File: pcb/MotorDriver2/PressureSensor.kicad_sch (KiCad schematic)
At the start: 22 parts, among them J2 Conn_01x02, J3 Conn_01x02, J4 Conn_01x02, J5 Conn_01x02, U6 LM324DR

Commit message: Laying out PCB
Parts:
- C_A1: LCSC (none) -> C77012
- R18, R19: LCSC (none) -> C25871
- U6: footprint footprintLib:D14 -> CapstoneFootprints:D14
- VR1, VR2, VR3, VR4: footprint footprintLib:TS53YJ105MR10 -> CapstoneFootprints:TS53YJ105MR10
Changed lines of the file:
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@@
 		(dnp no)
 		(fields_autoplaced yes)
-		(property "Reference" "#PWR065"
+		(property "Reference" "#PWR025"
 			(at 60.96 111.76 0)
 			(effects
@@
 			(project "MotorDriver1"
 				(path "/6e0510ec-6dbc-4bc1-a315-3680b1127a92/84d965bc-7f0b-4bc5-931c-8ce848efd12b"
-					(reference "#PWR065")
+					(reference "#PWR025")
 					(unit 1)
 				)
@@
 		(dnp no)
 		(fields_autoplaced yes)
-		(property "Reference" "#PWR042"
+		(property "Reference" "#PWR026"
 			(at 60.96 171.45 0)
 			(effects
@@
 			(project "MotorDriver1"
 				(path "/6e0510ec-6dbc-4bc1-a315-3680b1127a92/84d965bc-7f0b-4bc5-931c-8ce848efd12b"
-					(reference "#PWR042")
+					(reference "#PWR026")
 					(unit 1)
 				)
@@
 			)
 		)
+		(property "LCSC" "C25871"
+			(at 118.11 39.37 0)
+			(effects
+				(font
+					(size 1.27 1.27)
+				)
+				(hide yes)
+			)
+		)
 		(pin "2"
 		)
@@
 		(dnp no)
 		(fields_autoplaced yes)
-		(property "Reference" "#PWR062"
+		(property "Reference" "#PWR029"
 			(at 185.42 40.64 0)
 			(effects
@@
 			(project "MotorDriver1"
 				(path "/6e0510ec-6dbc-4bc1-a315-3680b1127a92/84d965bc-7f0b-4bc5-931c-8ce848efd12b"
-					(reference "#PWR062")
+					(reference "#PWR029")
 					(unit 1)
 				)
@@
 		(dnp no)
 		(fields_autoplaced yes)
-		(property "Reference" "#PWR064"
+		(property "Reference" "#PWR023"
 			(at 52.07 77.47 0)
 			(effects
@@
 			(project "MotorDriver1"
 				(path "/6e0510ec-6dbc-4bc1-a315-3680b1127a92/84d965bc-7f0b-4bc5-931c-8ce848efd12b"
-					(reference "#PWR064")
+					(reference "#PWR023")
 					(unit 1)
 				)
@@
 		(dnp no)
 		(fields_autoplaced yes)
-		(property "Reference" "#PWR041"
+		(property "Reference" "#PWR024"
 			(at 52.07 137.16 0)
 			(effects
@@
 			(project "MotorDriver1"
 				(path "/6e0510ec-6dbc-4bc1-a315-3680b1127a92/84d965bc-7f0b-4bc5-931c-8ce848efd12b"
-					(reference "#PWR041")
+					(reference "#PWR024")
 					(unit 1)
 				)
@@
 		(dnp no)
 		(fields_autoplaced yes)
-		(property "Reference" "#PWR043"
+		(property "Reference" "#PWR028"
 			(at 118.11 49.53 0)
 			(effects
@@
 			(project "MotorDriver1"
 				(path "/6e0510ec-6dbc-4bc1-a315-3680b1127a92/84d965bc-7f0b-4bc5-931c-8ce848efd12b"
-					(reference "#PWR043")
+					(reference "#PWR028")
 					(unit 1)
 				)
@@
 		(dnp no)
 		(fields_autoplaced yes)
-		(property "Reference" "#PWR040"
+		(property "Reference" "#PWR027"
 			(at 62.23 40.64 0)
 			(effects
@@
 			(project "MotorDriver1"
 				(path "/6e0510ec-6dbc-4bc1-a315-3680b1127a92/84d965bc-7f0b-4bc5-931c-8ce848efd12b"
-					(reference "#PWR040")
+					(reference "#PWR027")
 					(unit 1)
 				)
@@
 			)
 		)
-		(property "Footprint" "footprintLib:TS53YJ105MR10"
+		(property "Footprint" "CapstoneFootprints:TS53YJ105MR10"
 			(at 226.06 238.43 0)
 			(effects
@@
 		(dnp no)
 		(fields_autoplaced yes)
-		(property "Reference" "#PWR063"
+		(property "Reference" "#PWR032"
 			(at 241.3 49.53 0)
 			(effects
@@
 			(project "MotorDriver1"
 				(path "/6e0510ec-6dbc-4bc1-a315-3680b1127a92/84d965bc-7f0b-4bc5-931c-8ce848efd12b"
-					(reference "#PWR063")
+					(reference "#PWR032")
 					(unit 1)
 				)
@@
 			)
 		)
-		(property "Footprint" "footprintLib:D14"
+		(property "Footprint" "CapstoneFootprints:D14"
 			(at 162.56 106.68 0)
 			(effects
@@
 			)
 		)
+		(property "LCSC" "C25871"
+			(at 60.96 161.29 0)
+			(effects
+				(font
+					(size 1.27 1.27)
+				)
+				(hide yes)
+			)
+		)
 		(pin "2"
 		)
@@
 			)
 		)
+		(property "LCSC" "C77012"
+			(at 123.19 91.44 0)
+			(effects
+				(font
+					(size 1.27 1.27)
+				)
+				(hide yes)
+			)
+		)
 		(pin "2"
 		)
@@
 		(dnp no)
 		(fields_autoplaced yes)
-		(property "Reference" "#PWR044"
+		(property "Reference" "#PWR031"
 			(at 215.9 114.3 0)
 			(effects
@@
 			(project ""
 				(path "/6e0510ec-6dbc-4bc1-a315-3680b1127a92/84d965bc-7f0b-4bc5-931c-8ce848efd12b"
-					(reference "#PWR044")
+					(reference "#PWR031")
 					(unit 1)
 				)
@@
 		(dnp no)
 		(fields_autoplaced yes)
-		(property "Reference" "#PWR0101"
+		(property "Reference" "#PWR030"
 			(at 203.2 87.63 0)
 			(effects
@@
 			(project "MotorDriver1"
 				(path "/6e0510ec-6dbc-4bc1-a315-3680b1127a92/84d965bc-7f0b-4bc5-931c-8ce848efd12b"
-					(reference "#PWR0101")
+					(reference "#PWR030")
 					(unit 1)
 				)
@@
 			)
 		)
-		(property "Footprint" "footprintLib:TS53YJ105MR10"
+		(property "Footprint" "CapstoneFootprints:TS53YJ105MR10"
 			(at 231.14 197.79 0)
 			(effects
@@
 			)
 		)
-		(property "Footprint" "footprintLib:TS53YJ105MR10"
+		(property "Footprint" "CapstoneFootprints:TS53YJ105MR10"
 			(at 148.59 237.16 0)
 			(effects
@@
 			)
 		)
-		(property "Footprint" "footprintLib:TS53YJ105MR10"
+		(property "Footprint" "CapstoneFootprints:TS53YJ105MR10"
 			(at 133.35 197.79 0)
 			(effects

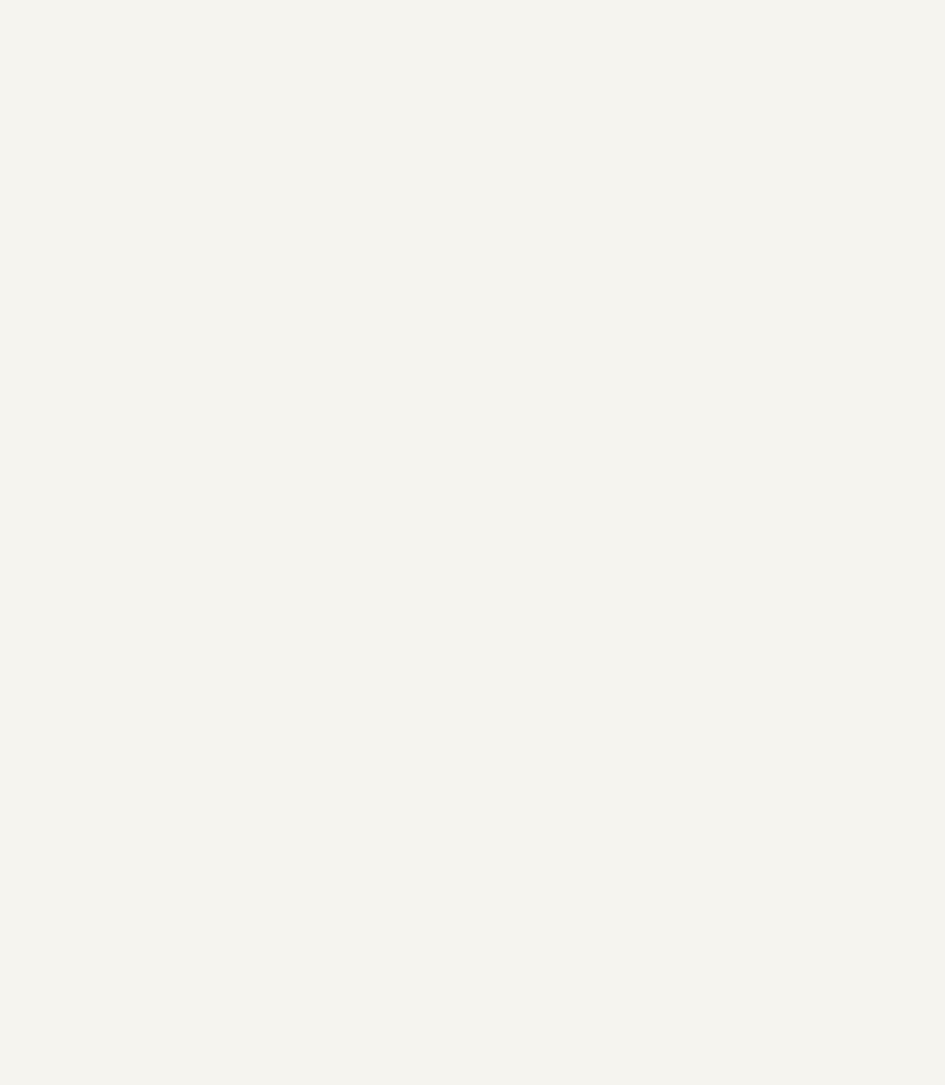
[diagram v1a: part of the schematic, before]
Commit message: Made some edits while making design poster
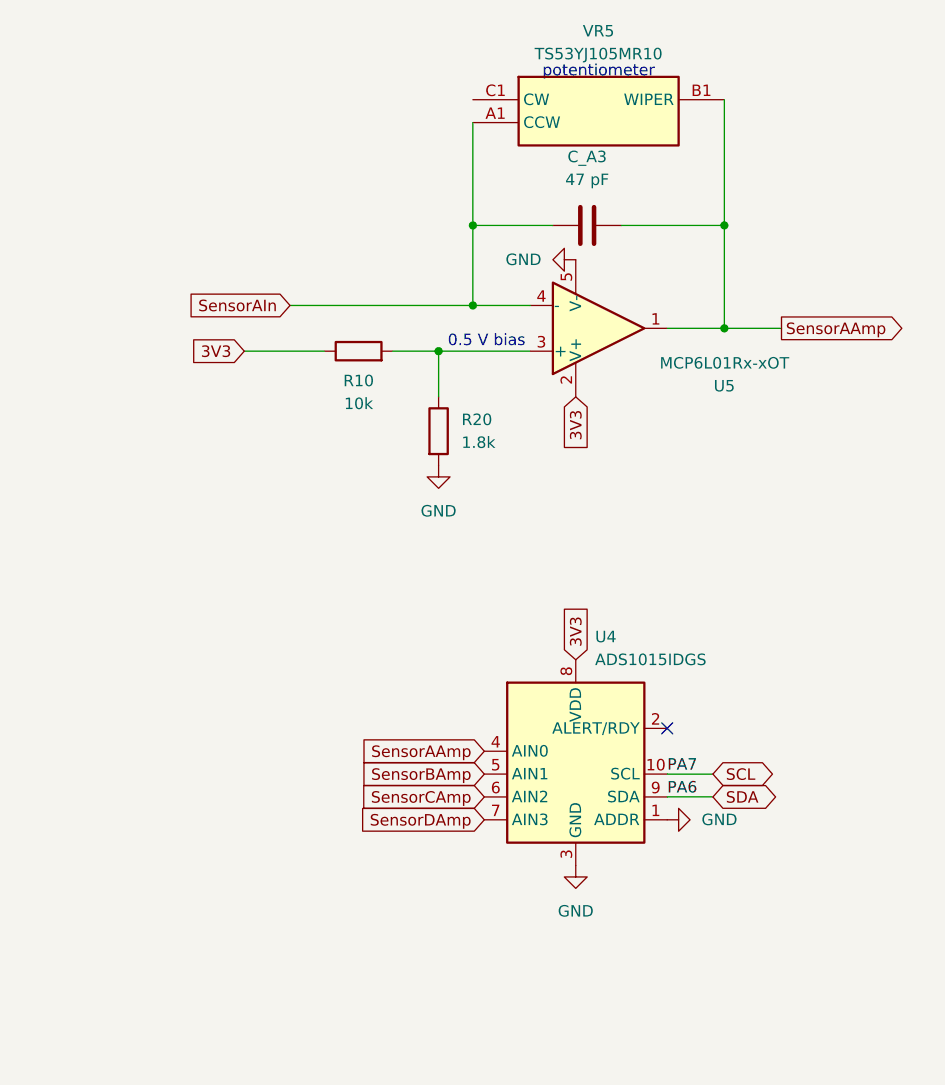
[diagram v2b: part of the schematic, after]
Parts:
- added C_A3: 47 pF, Capacitor_SMD:C_0402_1005Metric, symbol Device:C
- added R10: 10k, Resistor_SMD:R_0402_1005Metric, symbol Device:R
- added R20: 1.8k, Resistor_SMD:R_0402_1005Metric, symbol Device:R
- added U4: ADS1015IDGS, Package_SO:TSSOP-10_3x3mm_P0.5mm, symbol Analog_ADC:ADS1015IDGS
- added U5: MCP6L01Rx-xOT, Package_TO_SOT_SMD:SOT-23-5, symbol Amplifier_Operational:MCP6L01Rx-xOT
- added VR5: TS53YJ105MR10, CapstoneFootprints:TS53YJ105MR10, symbol pcb:TS53YJ105MR10
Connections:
- net 3V3: now also R10.1, U4.8 (VDD), U5.2 (V+)
- net GND: now also R20.2, U4.1 (ADDR), U4.3 (GND), U5.5 (V-)
- net SensorAIn: now also C_A3.2, U5.4 (-), VR5.A1 (CCW)
- new net: R10.2, R20.1, U5.3 (+)
- new net SCL: U4.10 (SCL)
- new net SDA: U4.9 (SDA)
- new net SensorAAmp: C_A3.1, U4.4 (AIN0), U5.1, VR5.B1 (WIPER)
- new net SensorBAmp: U4.5 (AIN1)
- new net SensorCAmp: U4.6 (AIN2)
- new net SensorDAmp: U4.7 (AIN3)
- no-connect marks 4 -> 5
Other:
- note added: "0.5 V bias"
- note added: "potentiometer"
